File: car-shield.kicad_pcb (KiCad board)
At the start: 2 copper layers, 66.7 x 64.1 mm, 35 parts

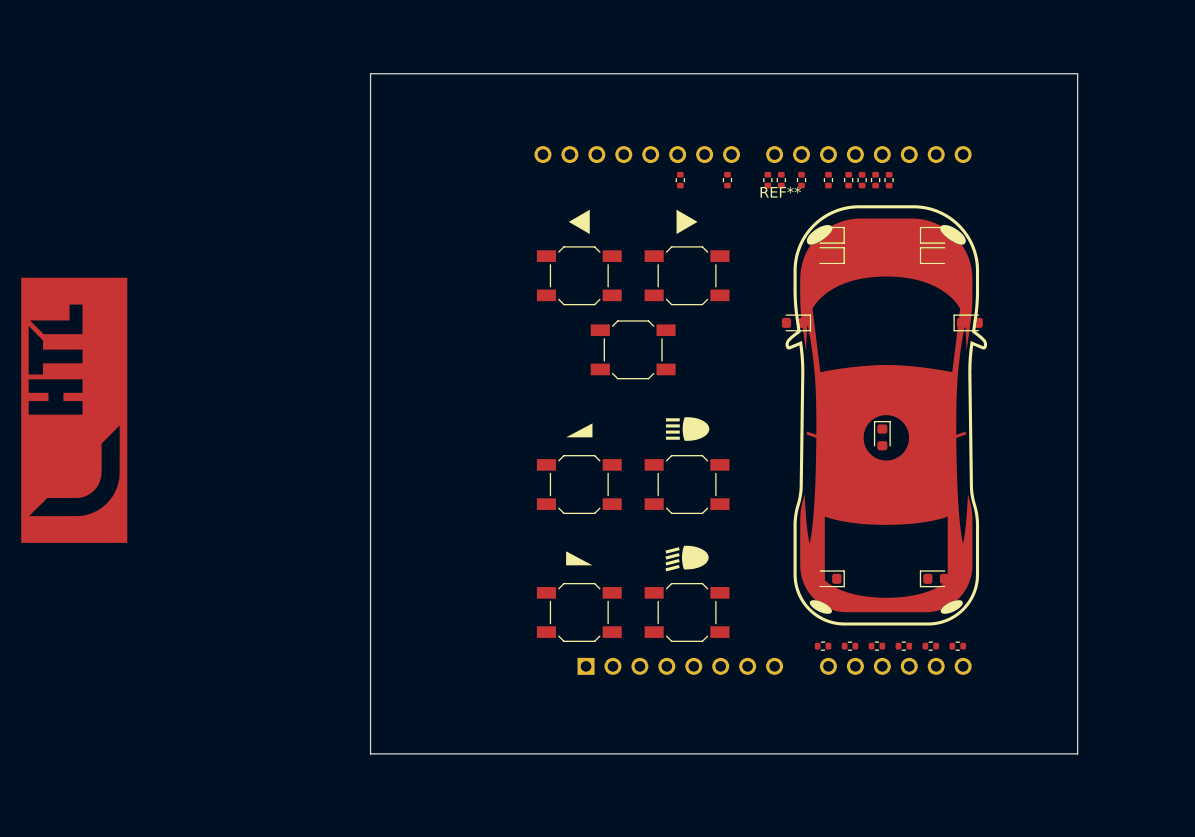
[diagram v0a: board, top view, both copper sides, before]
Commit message: some initial routing
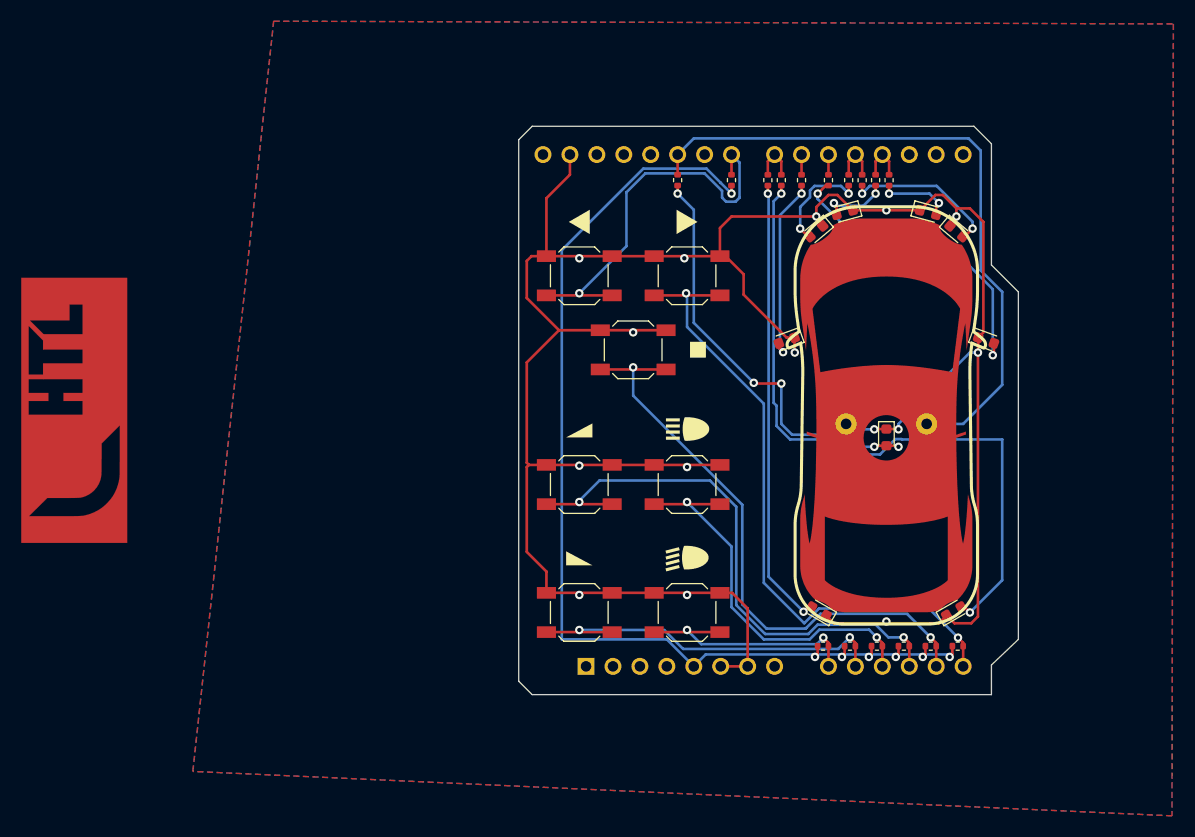
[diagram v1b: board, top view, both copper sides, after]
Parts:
- added BZ1: Buzzer, Buzzer_Beeper:Buzzer_15x7.5RM7.6, B.Cu at (159.1, 99.1)
- moved D8 3.47 mm to (161.7, 116.7), turned to 30 degrees
- moved D9 3.17 mm to (149.0, 116.7), turned to 150 degrees
- moved D4 2.98 mm to (161.9, 80.9), turned to -40 degrees
- moved D1 2.64 mm to (151.4, 79.1), turned to -165 degrees
- moved D3 2.56 mm to (148.7, 80.9), turned to -140 degrees
- moved D2 2.29 mm to (159.3, 79.1), turned to -15 degrees
- moved D6 2.25 mm to (164.7, 91.2), turned to -20 degrees
- moved D5 1.82 mm to (145.9, 91.2), turned to -160 degrees
- moved R10 0.38 mm to (140.7, 76.1)
- moved D7 0.38 mm to (155.3, 100.3)
- moved R7 0.25 mm to (135.6, 76.1)
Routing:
- net GND: track 0.00 -> 236.9 mm, vias 0 -> 15
- net VDD: track 0.00 -> 103.5 mm, vias 0 -> 7
- net Net-(D8-Pad2): track 0.00 -> 64.7 mm, vias 0 -> 2
- net speed_indicator: track 0.00 -> 63.2 mm
- net sw_right: track 0.00 -> 61.3 mm, vias 0 -> 2
- net sw_stop: track 0.00 -> 56.2 mm, vias 0 -> 2
- net sw_accel: track 0.00 -> 53.2 mm, vias 0 -> 2
- net Net-(D9-Pad2): track 0.00 -> 42.5 mm, vias 0 -> 2
- net Net-(D7-Pad2): track 0.00 -> 40.0 mm, vias 0 -> 5
- net sw_left: track 0.00 -> 37.1 mm, vias 0 -> 1
- net sw_high_b: track 0.00 -> 36.7 mm, vias 0 -> 2
- net sw_decel: track 0.00 -> 36.1 mm, vias 0 -> 2
- net Net-(D6-Pad2): track 0.00 -> 29.3 mm, vias 0 -> 2
- net sw_dipped_b: track 0.00 -> 23.0 mm, vias 0 -> 2
- net Net-(D5-Pad2): track 0.00 -> 17.7 mm, vias 0 -> 2
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- added copper zone on B.Cu, net GND
- added copper zone on F.Cu, net GND
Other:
- board size 66.7 x 64.1 mm -> 47.1 x 53.6 mm
